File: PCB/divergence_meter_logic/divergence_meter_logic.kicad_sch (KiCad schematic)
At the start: 16 parts

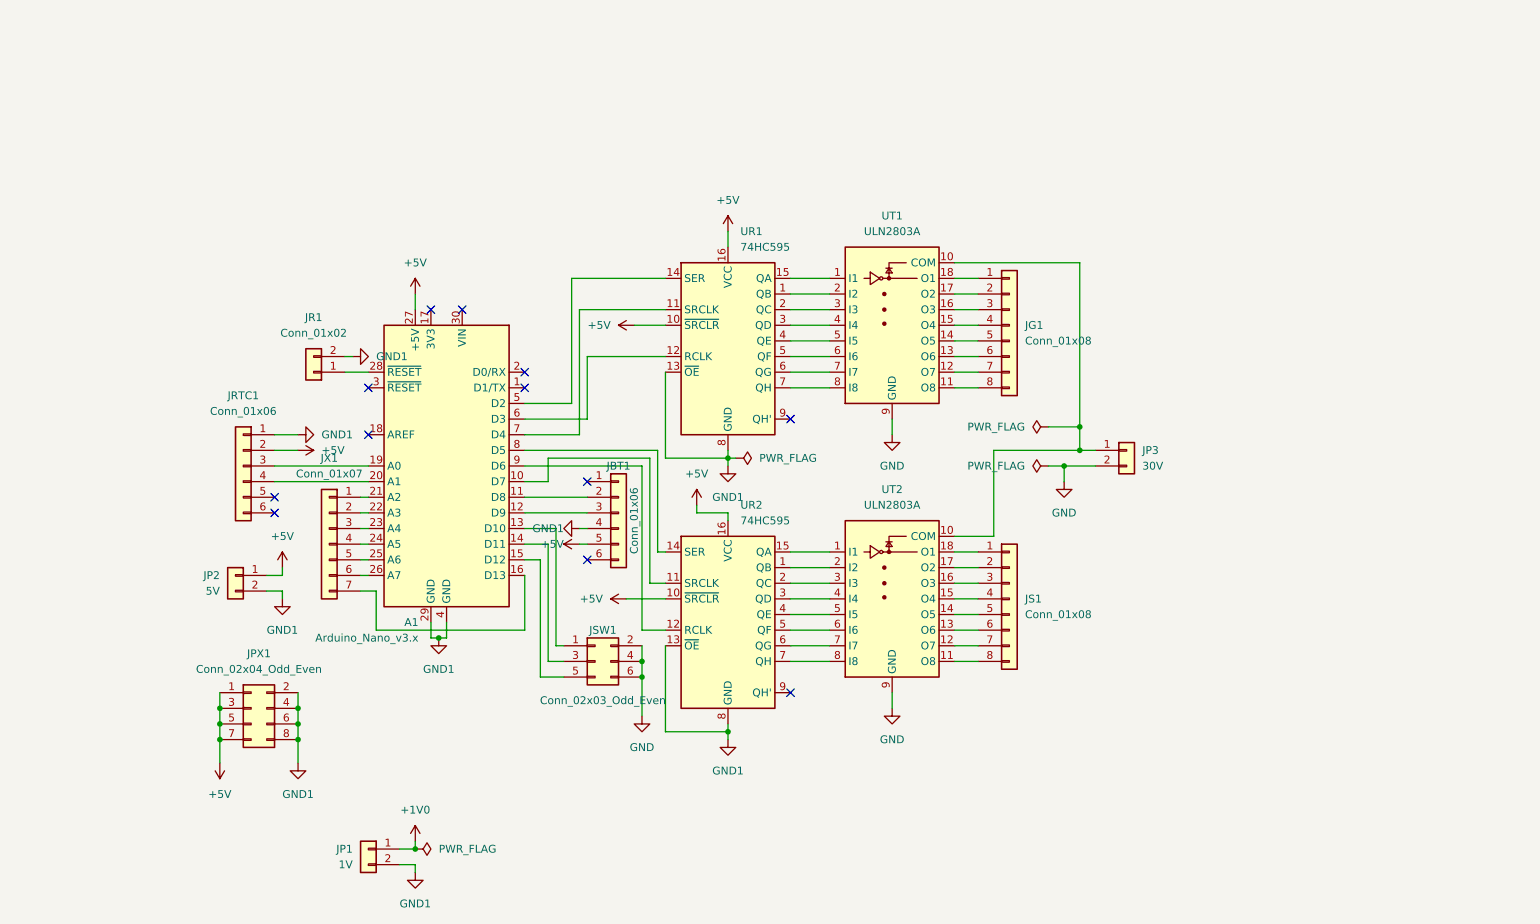
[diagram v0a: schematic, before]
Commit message: remake pcb
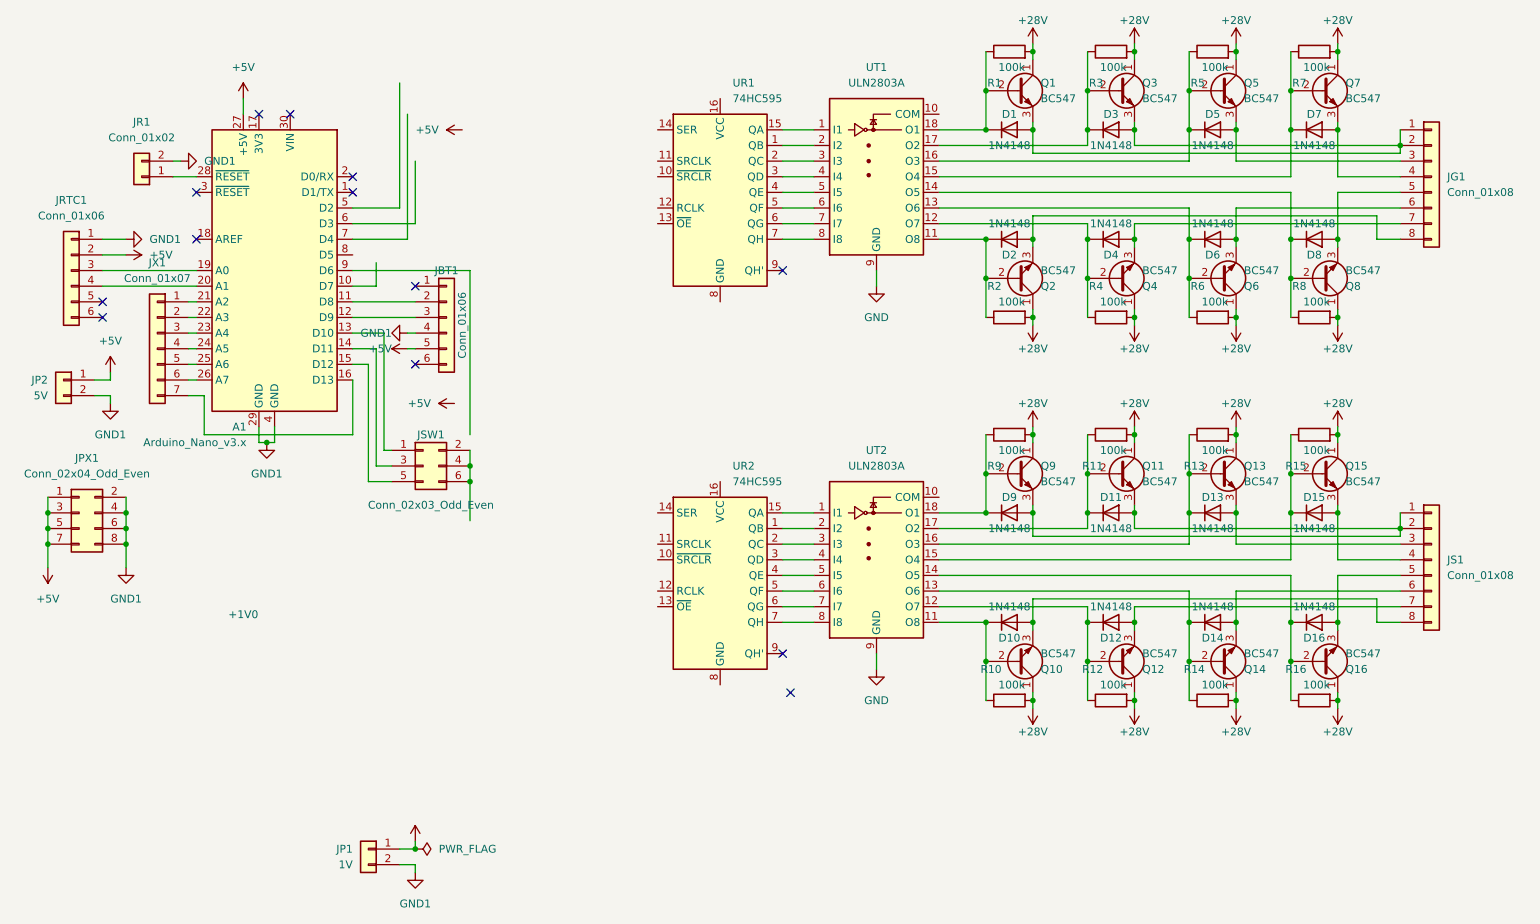
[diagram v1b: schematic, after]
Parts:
- removed JP3: 30V, symbol Connector_Generic:Conn_01x02
- added D1, D10, D11, D12, D13, D14, D15, D16, D2, D3, D4, D5, D6, D7, D8, D9: 1N4148, symbol Device:D
- added Q1, Q10, Q11, Q12, Q13, Q14, Q15, Q16, Q2, Q3, Q4, Q5, Q6, Q7, Q8, Q9: BC547, Package_TO_SOT_THT:TO-92_Inline, symbol Transistor_BJT:BC547
- added R1, R10, R11, R12, R13, R14, R15, R16, R2, R3, R4, R5, R6, R7, R8, R9: 100k, symbol Device:R
- JG1, JS1: footprint Connector_PinHeader_2.54mm:PinHeader_1x08_P2.54mm_Vertical -> Connector_PinSocket_2.54mm:PinSocket_1x08_P2.54mm_Vertical
- JRTC1: footprint Connector_PinHeader_2.54mm:PinHeader_1x06_P2.54mm_Vertical -> Connector_PinSocket_2.54mm:PinSocket_1x06_P2.54mm_Vertical
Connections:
- net +5V: no longer UR1.10 (~{SRCLR}), UR1.16 (VCC), UR2.10 (~{SRCLR}), UR2.16 (VCC)
- net GND: no longer JSW1.2 (Pin_2), JSW1.4 (Pin_4), JSW1.6 (Pin_6)
- net GND1: no longer UR1.13 (~{OE}), UR1.8 (GND), UR2.13 (~{OE}), UR2.8 (GND)
- net at UT1.10 (COM): no longer UT2.10 (COM)
- net at UT2.11 (O8): now also D10.1 (K), Q10.2 (B), R10.1; no longer JS1.8 (Pin_8)
- net at UT2.12 (O7): now also D12.1 (K), Q12.2 (B), R12.1; no longer JS1.7 (Pin_7)
- net at UT2.13 (O6): now also D14.1 (K), Q14.2 (B), R14.1; no longer JS1.6 (Pin_6)
- net at UT2.14 (O5): now also D16.1 (K), Q16.2 (B), R16.1; no longer JS1.5 (Pin_5)
- net at UT2.15 (O4): now also D15.1 (K), Q15.2 (B), R15.1; no longer JS1.4 (Pin_4)
- net at UT2.16 (O3): now also D13.1 (K), Q13.2 (B), R13.1; no longer JS1.3 (Pin_3)
- net at UT2.17 (O2): now also D11.1 (K), Q11.2 (B), R11.1; no longer JS1.2 (Pin_2)
- net at UT2.18 (O1): now also D9.1 (K), Q9.2 (B), R9.1; no longer JS1.1 (Pin_1)
- net at A1.10 (D7): no longer UR2.11 (SRCLK)
- net at A1.5 (D2): no longer UR1.14 (SER)
- net at A1.6 (D3): no longer UR1.12 (RCLK)
- net at A1.7 (D4): no longer UR1.11 (SRCLK)
- net at A1.8 (D5): no longer UR2.14 (SER)
- net at A1.9 (D6): no longer UR2.12 (RCLK)
- net at UT1.11 (O8): now also D2.1 (K), Q2.2 (B), R2.1; no longer JG1.8 (Pin_8)
- net at UT1.12 (O7): now also D4.1 (K), Q4.2 (B), R4.1; no longer JG1.7 (Pin_7)
- net at UT1.13 (O6): now also D6.1 (K), Q6.2 (B), R6.1; no longer JG1.6 (Pin_6)
- net at UT1.14 (O5): now also D8.1 (K), Q8.2 (B), R8.1; no longer JG1.5 (Pin_5)
- net at UT1.15 (O4): now also D7.1 (K), Q7.2 (B), R7.1; no longer JG1.4 (Pin_4)
- net at UT1.16 (O3): now also D5.1 (K), Q5.2 (B), R5.1; no longer JG1.3 (Pin_3)
- net at JG1.2 (Pin_2): now also JG1.1 (Pin_1), D1.2 (A), D3.2 (A), Q1.3 (E), Q3.3 (E); no longer UT1.17 (O2)
- net at UT1.18 (O1): now also D1.1 (K), Q1.2 (B), R1.1; no longer JG1.1 (Pin_1)
- new net: D4.2 (A), JG1.7 (Pin_7), Q4.3 (E)
- new net: D10.2 (A), JS1.8 (Pin_8), Q10.3 (E)
- new net: D12.2 (A), JS1.7 (Pin_7), Q12.3 (E)
- new net: D8.2 (A), JG1.5 (Pin_5), Q8.3 (E)
- new net: D11.2 (A), D9.2 (A), JS1.1 (Pin_1), JS1.2 (Pin_2), Q11.3 (E), Q9.3 (E)
- new net: D3.1 (K), Q3.2 (B), R3.1, UT1.17 (O2)
- new net: D6.2 (A), JG1.6 (Pin_6), Q6.3 (E)
- new net: D15.2 (A), JS1.4 (Pin_4), Q15.3 (E)
- new net: D2.2 (A), JG1.8 (Pin_8), Q2.3 (E)
- new net: D14.2 (A), JS1.6 (Pin_6), Q14.3 (E)
- new net: D7.2 (A), JG1.4 (Pin_4), Q7.3 (E)
- new net: D5.2 (A), JG1.3 (Pin_3), Q5.3 (E)
- new net: D13.2 (A), JS1.3 (Pin_3), Q13.3 (E)
- new net: D16.2 (A), JS1.5 (Pin_5), Q16.3 (E)
- new net: JSW1.2 (Pin_2), JSW1.4 (Pin_4), JSW1.6 (Pin_6)
- new net +28V: Q1.1 (C), Q10.1 (C), Q11.1 (C), Q12.1 (C), Q13.1 (C), Q14.1 (C), Q15.1 (C), Q16.1 (C), Q2.1 (C), Q3.1 (C), Q4.1 (C), Q5.1 (C), Q6.1 (C), Q7.1 (C), Q8.1 (C), Q9.1 (C), R1.2, R10.2, R11.2, R12.2, R13.2, R14.2, R15.2, R16.2, R2.2, R3.2, R4.2, R5.2, R6.2, R7.2, R8.2, R9.2
- no-connect marks 12 -> 13
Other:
- moved on the sheet: A1, JBT1, JG1, JP2, JPX1, JR1, JRTC1, JSW1, JX1, UR1, UT1
